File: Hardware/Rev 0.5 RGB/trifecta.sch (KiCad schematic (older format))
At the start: 284 parts, among them J1 USB2_C_Receptacle, SW1 RESET, SW2 Rotary_Encoder_Switch, SW3 Rotary_Encoder_Switch, SW4 Rotary_Encoder_Switch, U1 ATmega32U4-AU, U2 SRV05-4, Y1 16MHz

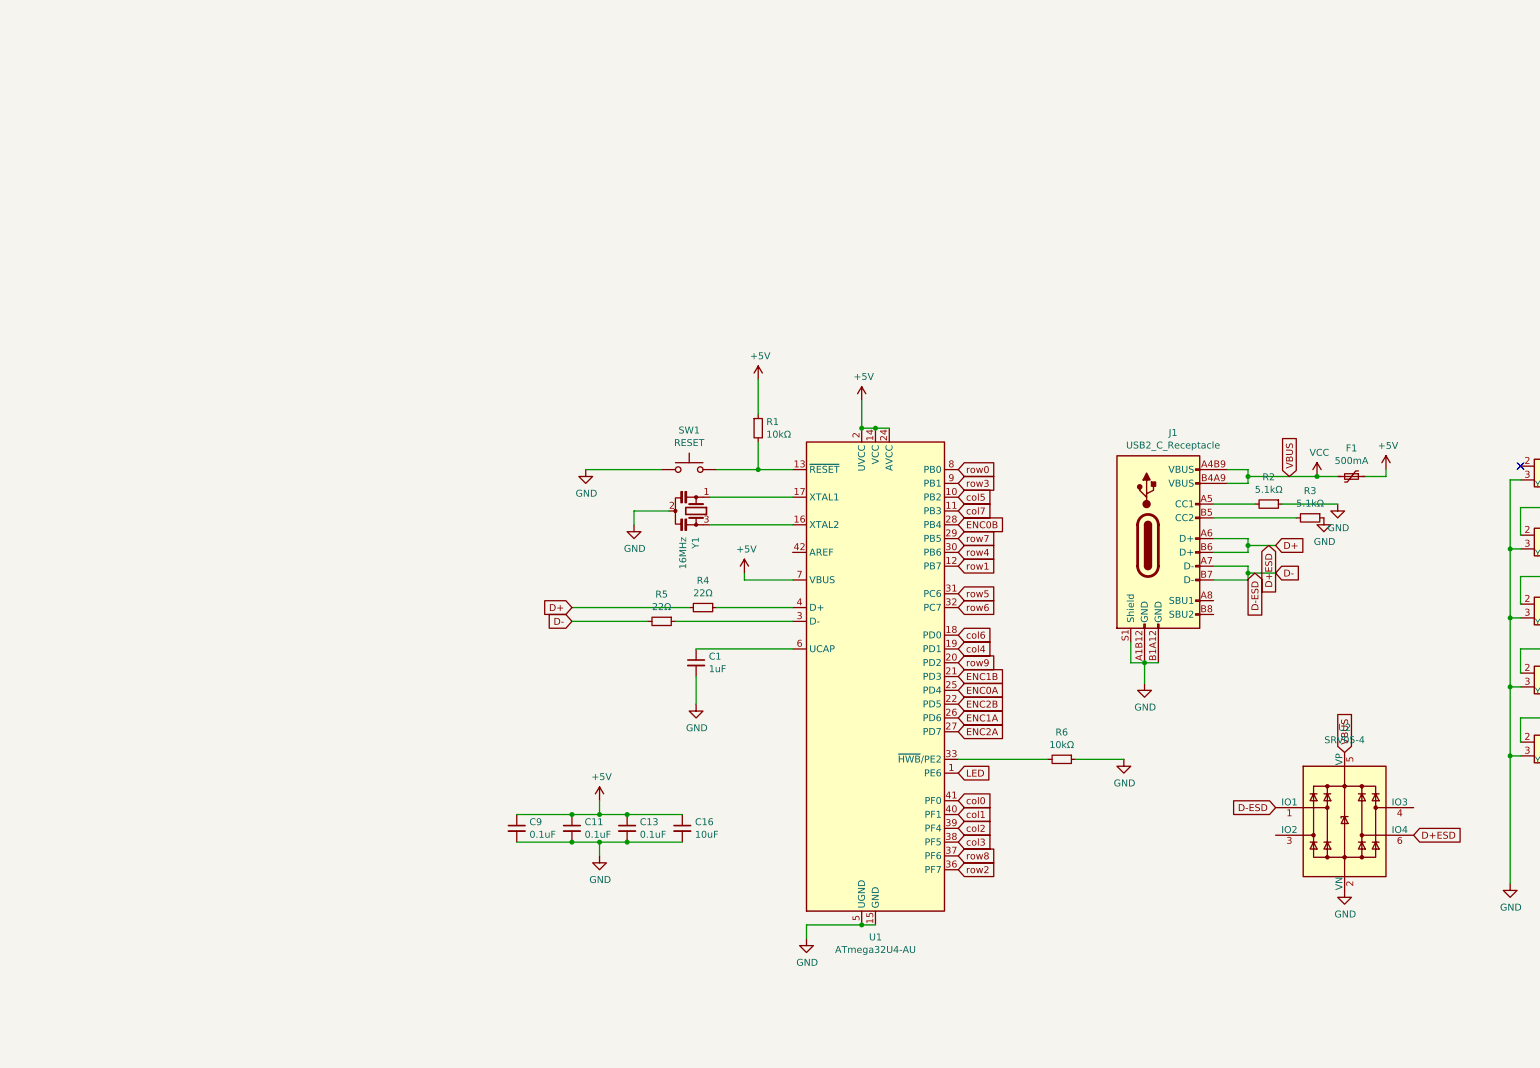
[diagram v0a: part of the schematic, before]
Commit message: 8/8
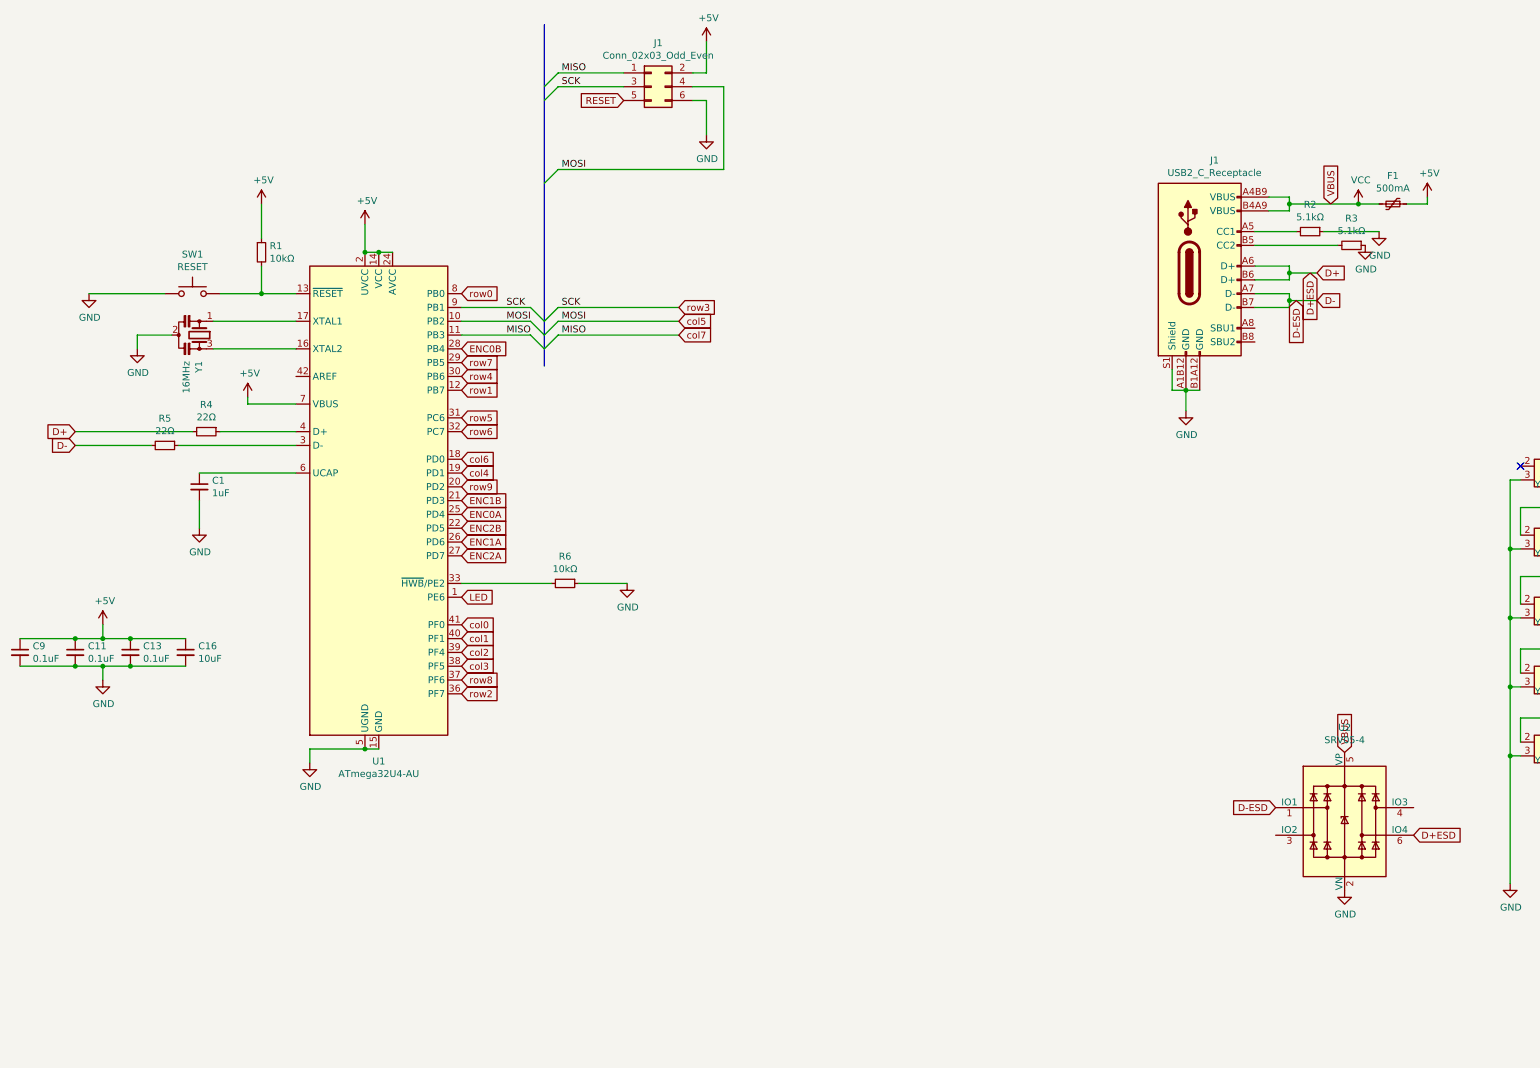
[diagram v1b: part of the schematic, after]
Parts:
- added J1: Conn_02x03_Odd_Even, Connector_PinHeader_2.54mm:PinHeader_2x03_P2.54mm_Vertical, symbol conn:Conn_02x03_Odd_Even
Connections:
- net +5V: now also J1.2 (Pin_2)
- net 0col: now also J1.1 (Pin_1)
- net GND: now also J1.6 (Pin_6)
- net col5: now also J1.4 (Pin_4)
- net row3: now also J1.3 (Pin_3)
- new net RESET: J1.5 (Pin_5)
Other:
- moved on the sheet: C1, C11, C13, C16, C9, F1, J1, R1, R2, R3, R4, R5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
